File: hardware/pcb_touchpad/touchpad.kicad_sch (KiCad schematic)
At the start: 23 parts

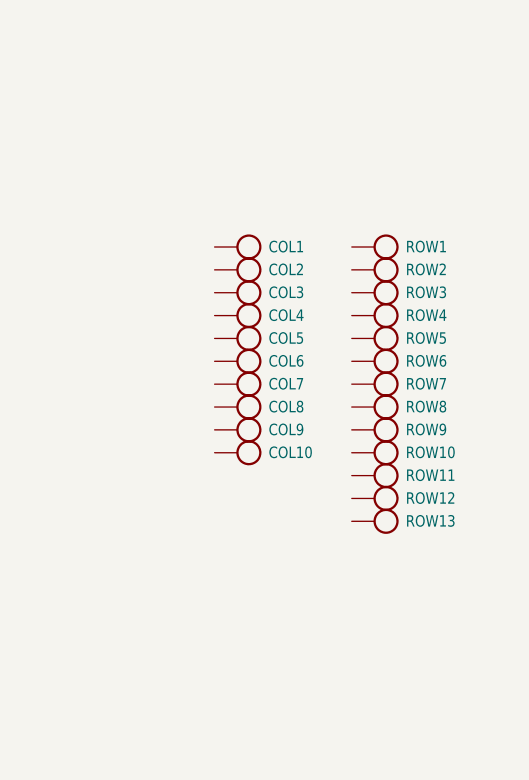
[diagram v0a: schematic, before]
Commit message: created iqs9151 symbol
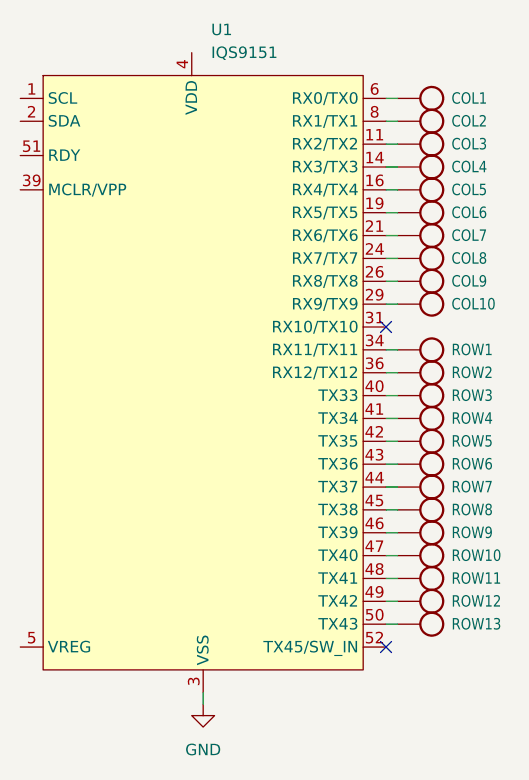
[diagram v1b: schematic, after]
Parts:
- added U1: IQS9151, Package_DFN_QFN:VQFN-52-1EP_6x6mm_P0.4mm_EP4.7x4.7mm, symbol IQS9151:IQS9151
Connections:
- net at ROW7.P1: now also U1.44 (TX37)
- net at COL10.P1: now also U1.29 (RX9/TX9)
- net at ROW2.P1: now also U1.36 (RX12/TX12)
- net at ROW11.P1: now also U1.48 (TX41)
- net at COL9.P1: now also U1.26 (RX8/TX8)
- net at COL3.P1: now also U1.11 (RX2/TX2)
- net at COL5.P1: now also U1.16 (RX4/TX4)
- net at ROW8.P1: now also U1.45 (TX38)
- net at ROW6.P1: now also U1.43 (TX36)
- net at COL8.P1: now also U1.24 (RX7/TX7)
- net at ROW10.P1: now also U1.47 (TX40)
- net at COL7.P1: now also U1.21 (RX6/TX6)
- net at ROW1.P1: now also U1.34 (RX11/TX11)
- net at ROW9.P1: now also U1.46 (TX39)
- net at COL4.P1: now also U1.14 (RX3/TX3)
- net at ROW13.P1: now also U1.50 (TX43)
- net at ROW3.P1: now also U1.40 (TX33)
- net at ROW5.P1: now also U1.42 (TX35)
- net at ROW12.P1: now also U1.49 (TX42)
- net at ROW4.P1: now also U1.41 (TX34)
- net at COL1.P1: now also U1.6 (RX0/TX0)
- net at COL2.P1: now also U1.8 (RX1/TX1)
- net at COL6.P1: now also U1.19 (RX5/TX5)
- new net: U1.37 (NC), U1.38 (NC)
- new net GND: U1.3 (VSS)
- no-connect marks 0 -> 2
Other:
- moved on the sheet: COL1, COL10, COL2, COL3, COL4, COL5, COL6, COL7, COL8, COL9, ROW1, ROW10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
